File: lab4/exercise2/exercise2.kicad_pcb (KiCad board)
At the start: 2 copper layers, 40.6 x 38.1 mm, 10 parts, among them J1 Conn_01x02_Male, U1 NE555D

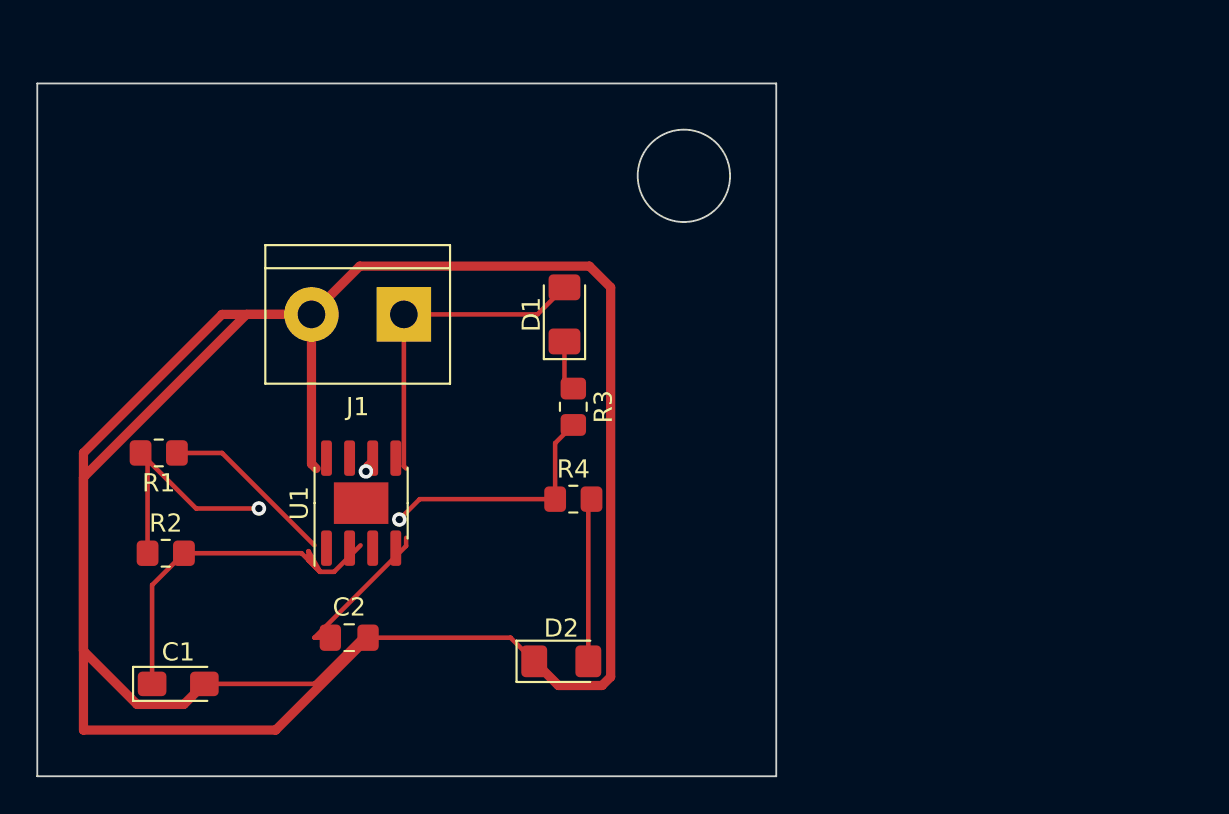
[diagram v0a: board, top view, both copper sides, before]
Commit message: pcb update
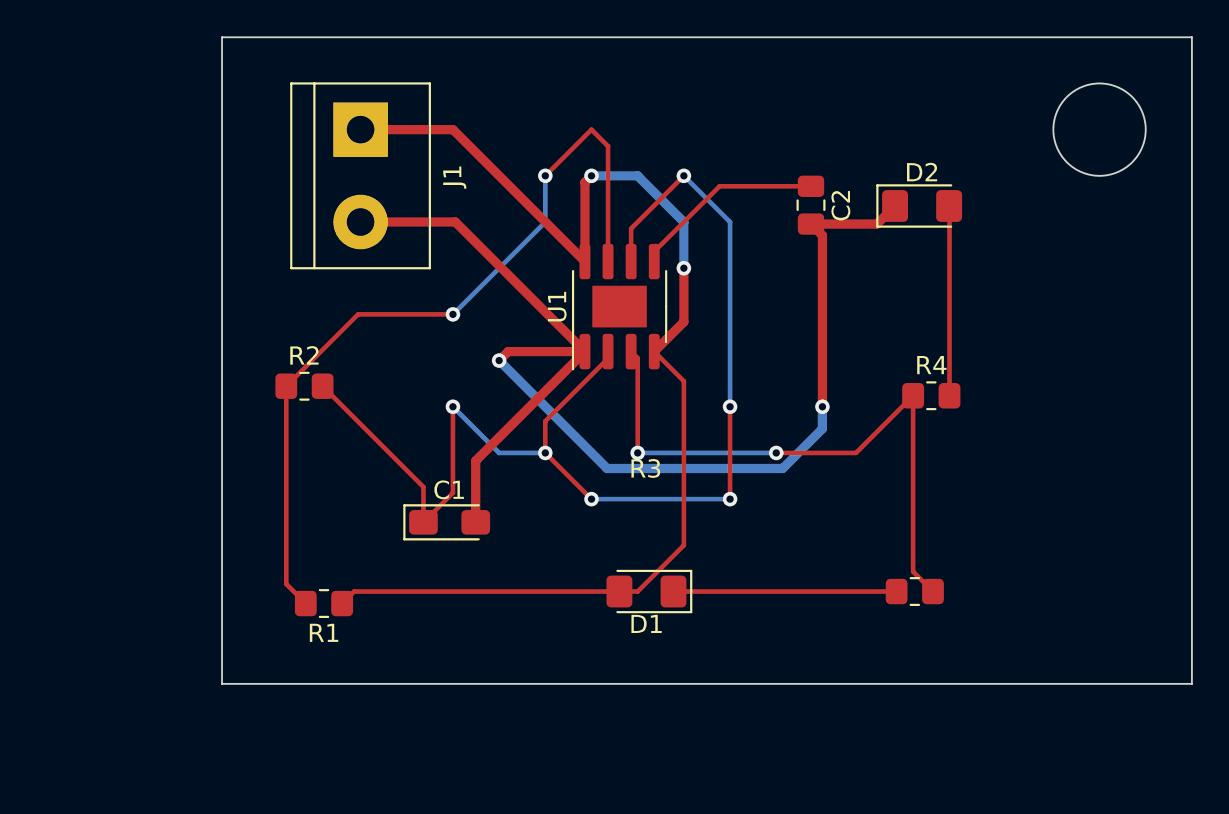
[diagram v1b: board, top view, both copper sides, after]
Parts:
- moved C2 34.8 mm to (146.7, 70.2), turned to -90 degrees
- moved D2 31.9 mm to (152.8, 70.2)
- moved R3 21.4 mm to (152.4, 91.4), turned to 0 degrees
- moved R4 20.5 mm to (153.3, 80.7)
- moved U1 17.9 mm to (136.2, 75.8)
- moved C1 17.4 mm to (126.8, 87.6)
- moved D1 15.9 mm to (137.6, 91.4), turned to 180 degrees
- moved R1 12.3 mm to (119.9, 92.1)
- moved R2 11.9 mm to (118.8, 80.2)
- moved J1 10.4 mm to (121.9, 66.0), turned to -90 degrees
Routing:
- net GND: track 155.5 -> 69.8 mm, vias 0 -> 2
- net /pin_2: track 22.2 -> 65.9 mm, vias 1 -> 6
- net +9V: track 27.6 -> 65.6 mm, vias 0 -> 2
- net /pin_7: track 13.4 -> 44.1 mm, vias 1 -> 2
- net /pin_3: track 13.5 -> 33.4 mm, vias 1 -> 2
- net Net-(D1-Pad1): track 2.79 -> 12.3 mm
- net Net-(C2-Pad1): track 8.46 -> 10.7 mm
- net Net-(D2-Pad2): track 8.99 -> 10.4 mm
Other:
- board size 40.6 x 38.1 mm -> 53.3 x 35.6 mm
